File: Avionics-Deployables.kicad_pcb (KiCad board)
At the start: 2 copper layers, 82 x 100 mm, 27 parts, among them J1 200528-0100

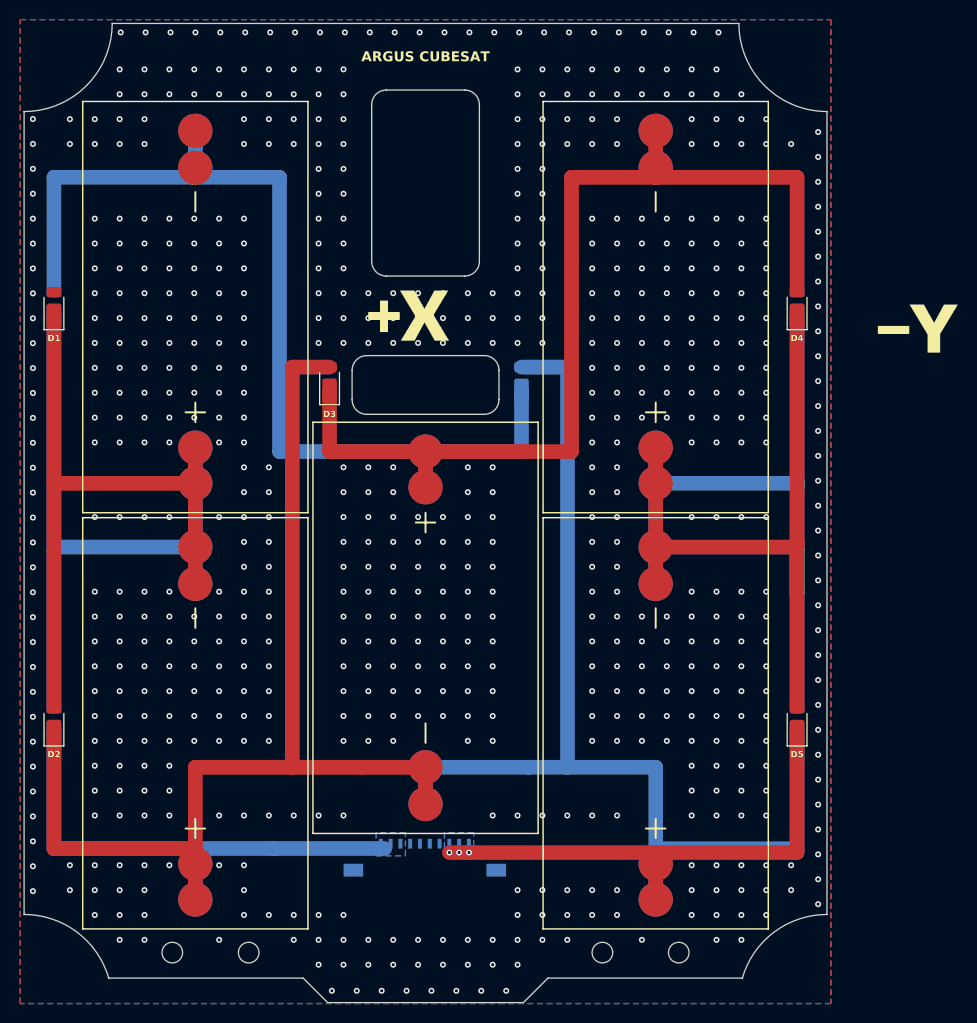
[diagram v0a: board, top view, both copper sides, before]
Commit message: V3 Updates and Cell Backer
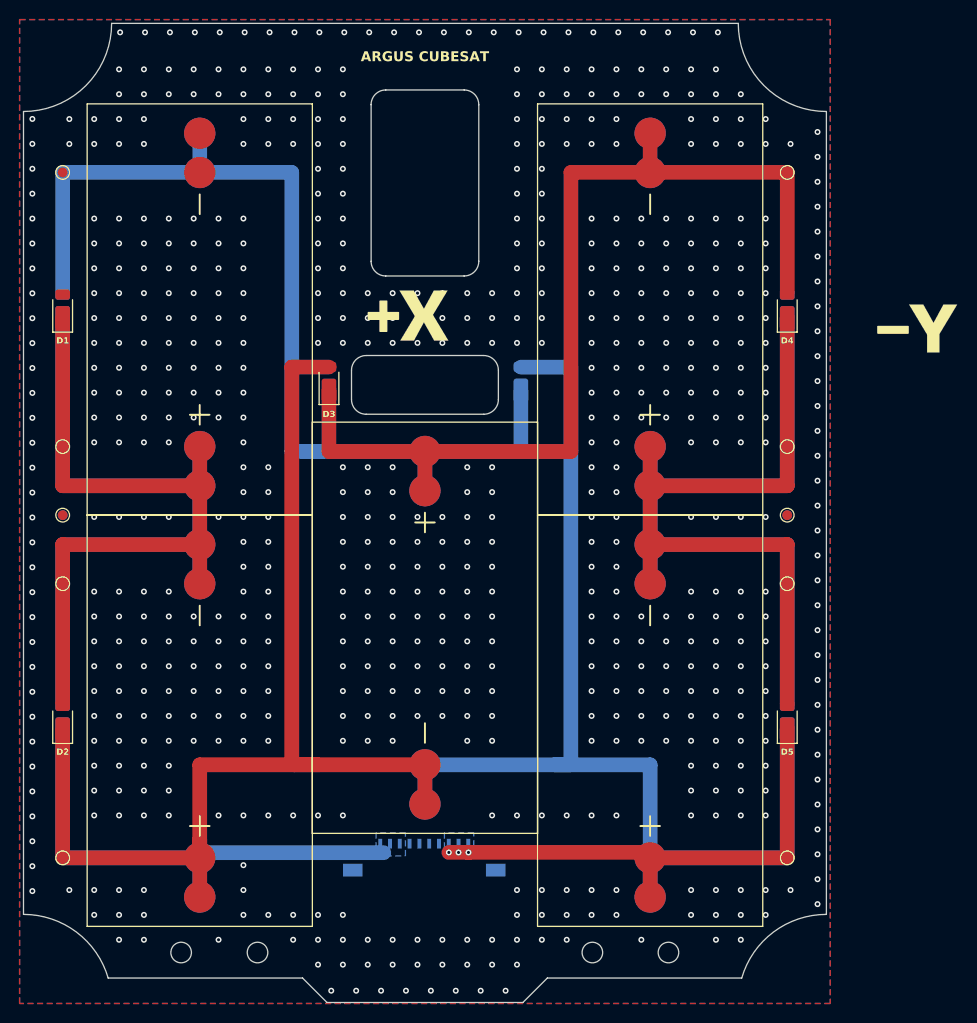
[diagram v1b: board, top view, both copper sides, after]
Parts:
- added H1: MountingHole_Pad, TestPoint:TestPoint_Pad_D1.0mm, F.Cu at (109.6, 84.6)
- added H10: MountingHole_Pad, TestPoint:TestPoint_Pad_D1.0mm, B.Cu at (183.6, 84.6)
- added H11: MountingHole_Pad, TestPoint:TestPoint_Pad_D1.0mm, B.Cu at (183.6, 126.6)
- added H12: MountingHole_Pad, TestPoint:TestPoint_Pad_D1.0mm, B.Cu at (109.6, 56.6)
- added H13: MountingHole_Pad, TestPoint:TestPoint_Pad_D1.0mm, B.Cu at (109.6, 84.6)
- added H14: MountingHole_Pad, TestPoint:TestPoint_Pad_D1.0mm, B.Cu at (109.6, 126.6)
- added H15: MountingHole_Pad, TestPoint:TestPoint_Pad_D1.0mm, B.Cu at (183.6, 98.6)
- added H16: MountingHole_Pad, TestPoint:TestPoint_Pad_D1.0mm, B.Cu at (109.6, 98.6)
- added H17: MountingHole_Pad, TestPoint:TestPoint_Pad_D1.0mm, B.Cu at (183.6, 91.6)
- added H18: MountingHole_Pad, TestPoint:TestPoint_Pad_D1.0mm, B.Cu at (109.6, 91.6)
- added H19: MountingHole_Pad, TestPoint:TestPoint_Pad_D1.0mm, F.Cu at (183.6, 91.6)
- added H2: MountingHole_Pad, TestPoint:TestPoint_Pad_D1.0mm, F.Cu at (183.6, 84.6)
- added H20: MountingHole_Pad, TestPoint:TestPoint_Pad_D1.0mm, F.Cu at (109.6, 91.6)
- added H3: MountingHole_Pad, TestPoint:TestPoint_Pad_D1.0mm, F.Cu at (109.6, 56.6)
- added H4: MountingHole_Pad, TestPoint:TestPoint_Pad_D1.0mm, F.Cu at (109.6, 98.6)
- added H5: MountingHole_Pad, TestPoint:TestPoint_Pad_D1.0mm, F.Cu at (109.6, 126.6)
- added H6: MountingHole_Pad, TestPoint:TestPoint_Pad_D1.0mm, F.Cu at (183.6, 56.6)
- added H7: MountingHole_Pad, TestPoint:TestPoint_Pad_D1.0mm, F.Cu at (183.6, 98.6)
- added H8: MountingHole_Pad, TestPoint:TestPoint_Pad_D1.0mm, F.Cu at (183.6, 126.6)
- added H9: MountingHole_Pad, TestPoint:TestPoint_Pad_D1.0mm, B.Cu at (183.6, 56.6)
- D1, D10, D2, D3, D4, D5, D6, D7, D8, D9: value DFLS130L-7 -> DFLS130LQ-7
- SC1, SC10, SC2, SC3, SC4, SC5, SC6, SC7, SC8, SC9: footprint SolarPanels:SM141K06TF-S -> Argus-Miscellaneous:SM141K06TF_S
- moved D5 1.04 mm to (183.6, 112.6)
- moved D7 1.04 mm to (183.6, 112.6)
- moved D4 1.04 mm to (183.6, 70.6)
- moved D6 1.04 mm to (183.6, 70.6)
- moved D10 0.93 mm to (109.6, 112.6)
- moved D2 0.93 mm to (109.6, 112.6)
- moved D1 0.92 mm to (109.6, 70.6)
- moved D9 0.92 mm to (109.6, 70.6)
- moved SC5 0.62 mm to (169.6, 112.6)
- moved SC7 0.62 mm to (169.6, 112.6)
- moved SC4 0.62 mm to (169.6, 70.6)
- moved SC6 0.62 mm to (169.6, 70.6)
- moved SC10 0.52 mm to (123.6, 112.6)
- moved SC2 0.52 mm to (123.6, 112.6)
- moved SC1 0.51 mm to (123.6, 70.6)
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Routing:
- net Net-(D1-K): track 67.1 -> 75.1 mm
- net Net-(D4-K): track 68.4 -> 75.7 mm
- net Net-(D10-A): track 68.4 -> 75.5 mm
- net Net-(D2-K): track 111.8 -> 116.7 mm
- net Net-(D8-K): track 102.0 -> 106.2 mm
- net Net-(D6-K): track 73.6 -> 75.1 mm
- net D_VSOLAR2: track 50.9 -> 50.0 mm
- net Net-(D7-K): track 115.8 -> 115.2 mm
- net Net-(D3-K): track 101.9 -> 101.4 mm
- net GND: vias 693 -> 680
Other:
- outline, holes or cut-outs redrawn
